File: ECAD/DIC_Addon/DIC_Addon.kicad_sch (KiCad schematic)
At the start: 86 parts, among them J1 WE 62702621621, J3 WE 62702621621, Q1 FDN352AP, Q10 2N7002, Q11 FDN352AP, Q12 2N7002, Q13 FDN352AP, Q14 FDN352AP, Q15 2N7002, Q16 FDN352AP, Q17 FDN352AP, Q18 2N7002, Q2 FDN352AP, Q3 2N7002, Q4 FDN352AP, Q5 FDN352AP, Q6 2N7002, Q7 FDN352AP, Q8 FDN352AP, Q9 FDN352AP

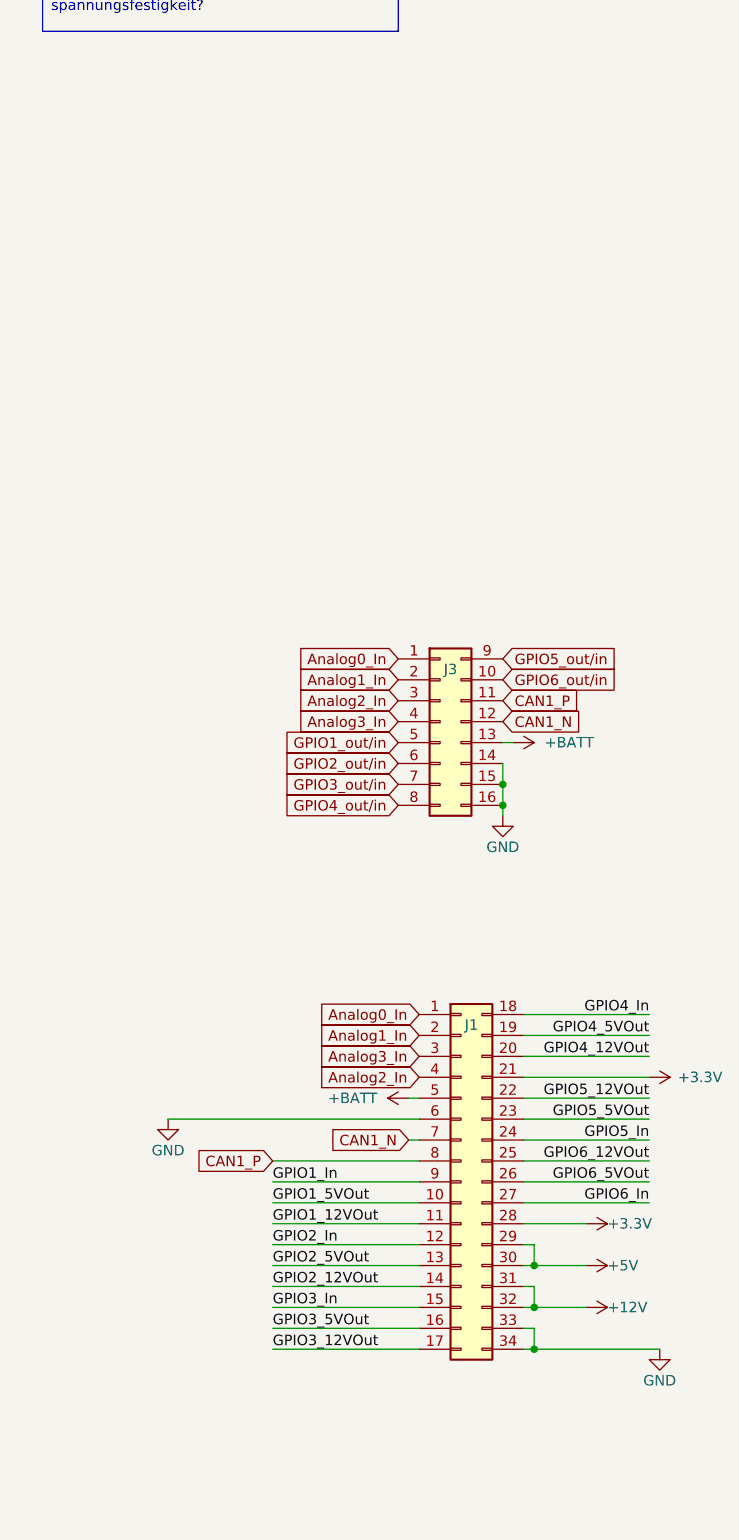
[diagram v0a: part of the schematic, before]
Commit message: finisjed PCB projekt
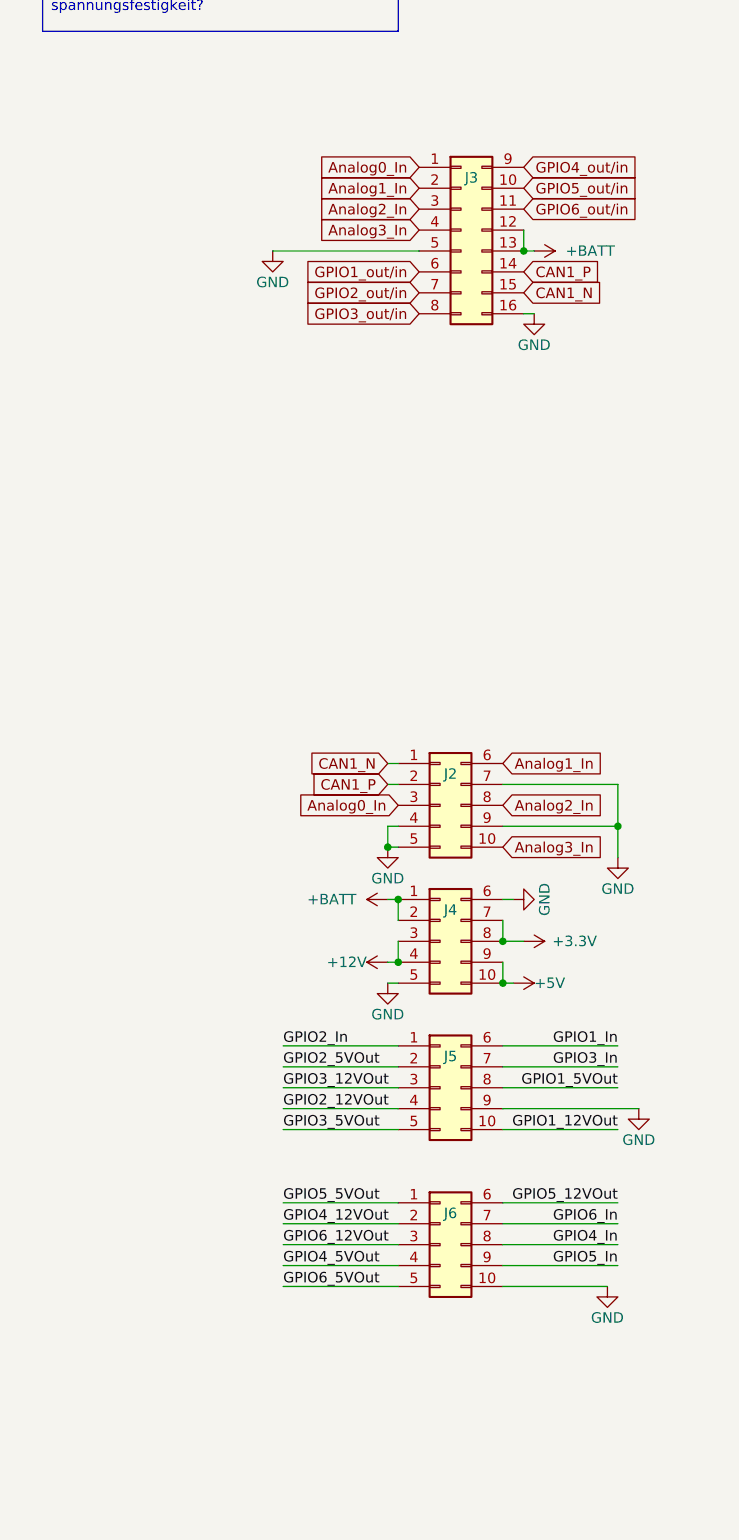
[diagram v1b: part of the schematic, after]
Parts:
- removed J1: WE 62702621621, Connector_PinHeader_1.27mm:PinHeader_2x17_P1.27mm_Vertical, symbol Connector_Generic:Conn_02x17_Top_Bottom
- added J2, J4, J5, J6: Conn_02x05_Top_Bottom, Connector_PinSocket_1.27mm:PinSocket_2x05_P1.27mm_Vertical, symbol Connector_Generic:Conn_02x05_Top_Bottom
- J3: footprint Connector_PinHeader_1.27mm:PinHeader_2x07_P1.27mm_Vertical -> Connector_PinHeader_1.27mm:PinHeader_2x08_P1.27mm_Vertical
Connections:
- net +12V: now also J4.3 (Pin_3), J4.4 (Pin_4)
- net +3.3V: now also J4.7 (Pin_7), J4.8 (Pin_8)
- net +5V: now also J4.10 (Pin_10), J4.9 (Pin_9)
- net +BATT: now also J3.12 (Pin_12), J4.1 (Pin_1), J4.2 (Pin_2)
- net Analog0_In: now also J2.3 (Pin_3)
- net Analog1_In: now also J2.6 (Pin_6)
- net Analog2_In: now also J2.8 (Pin_8)
- net Analog3_In: now also J2.10 (Pin_10)
- net CAN1_N: now also J3.15 (Pin_15), J2.1 (Pin_1); no longer J3.12 (Pin_12)
- net CAN1_P: now also J3.14 (Pin_14), J2.2 (Pin_2); no longer J3.11 (Pin_11)
- net GND: now also J3.5 (Pin_5), J2.4 (Pin_4), J2.5 (Pin_5), J2.7 (Pin_7), J2.9 (Pin_9), J4.5 (Pin_5), J4.6 (Pin_6), J5.9 (Pin_9), J6.10 (Pin_10); no longer J3.14 (Pin_14), J3.15 (Pin_15)
- net GPIO1_12VOut: now also J5.10 (Pin_10)
- net GPIO1_5VOut: now also J5.8 (Pin_8)
- net GPIO1_In: now also J5.6 (Pin_6)
- net GPIO1_out/in: now also J3.6 (Pin_6); no longer J3.5 (Pin_5)
- net GPIO2_12VOut: now also J5.4 (Pin_4)
- net GPIO2_5VOut: now also J5.2 (Pin_2)
- net GPIO2_In: now also J5.1 (Pin_1)
- net GPIO2_out/in: now also J3.7 (Pin_7); no longer J3.6 (Pin_6)
- net GPIO3_12VOut: now also J5.3 (Pin_3)
- net GPIO3_5VOut: now also J5.5 (Pin_5)
- net GPIO3_In: now also J5.7 (Pin_7)
- net GPIO3_out/in: now also J3.8 (Pin_8); no longer J3.7 (Pin_7)
- net GPIO4_12VOut: now also J6.2 (Pin_2)
- net GPIO4_5VOut: now also J6.4 (Pin_4)
- net GPIO4_In: now also J6.8 (Pin_8)
- net GPIO4_out/in: now also J3.9 (Pin_9); no longer J3.8 (Pin_8)
- net GPIO5_12VOut: now also J6.6 (Pin_6)
- net GPIO5_5VOut: now also J6.1 (Pin_1)
- net GPIO5_In: now also J6.9 (Pin_9)
- net GPIO5_out/in: now also J3.10 (Pin_10); no longer J3.9 (Pin_9)
- net GPIO6_12VOut: now also J6.3 (Pin_3)
- net GPIO6_5VOut: now also J6.5 (Pin_5)
- net GPIO6_In: now also J6.7 (Pin_7)
- net GPIO6_out/in: now also J3.11 (Pin_11); no longer J3.10 (Pin_10)
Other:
- moved on the sheet: J3
